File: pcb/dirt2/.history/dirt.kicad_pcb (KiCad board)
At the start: 2 copper layers, 1 part

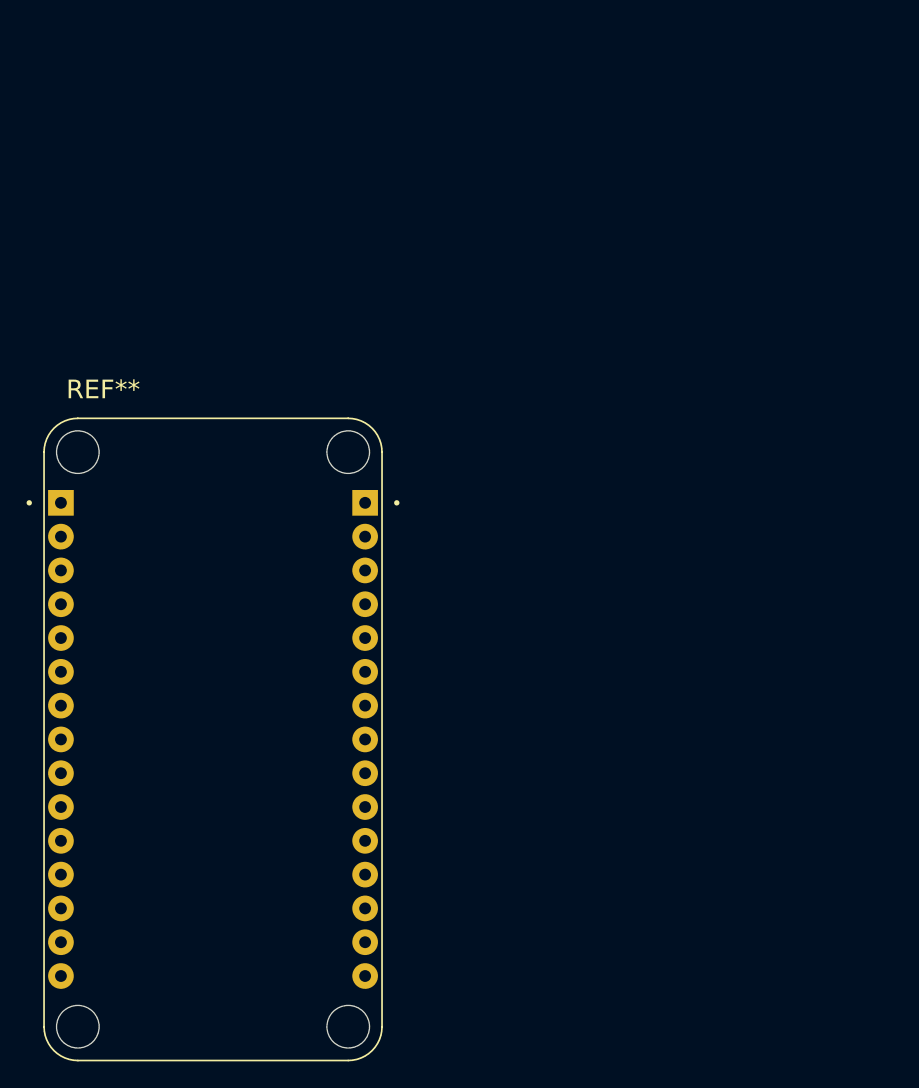
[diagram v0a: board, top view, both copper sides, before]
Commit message: i created some edits and added the zine
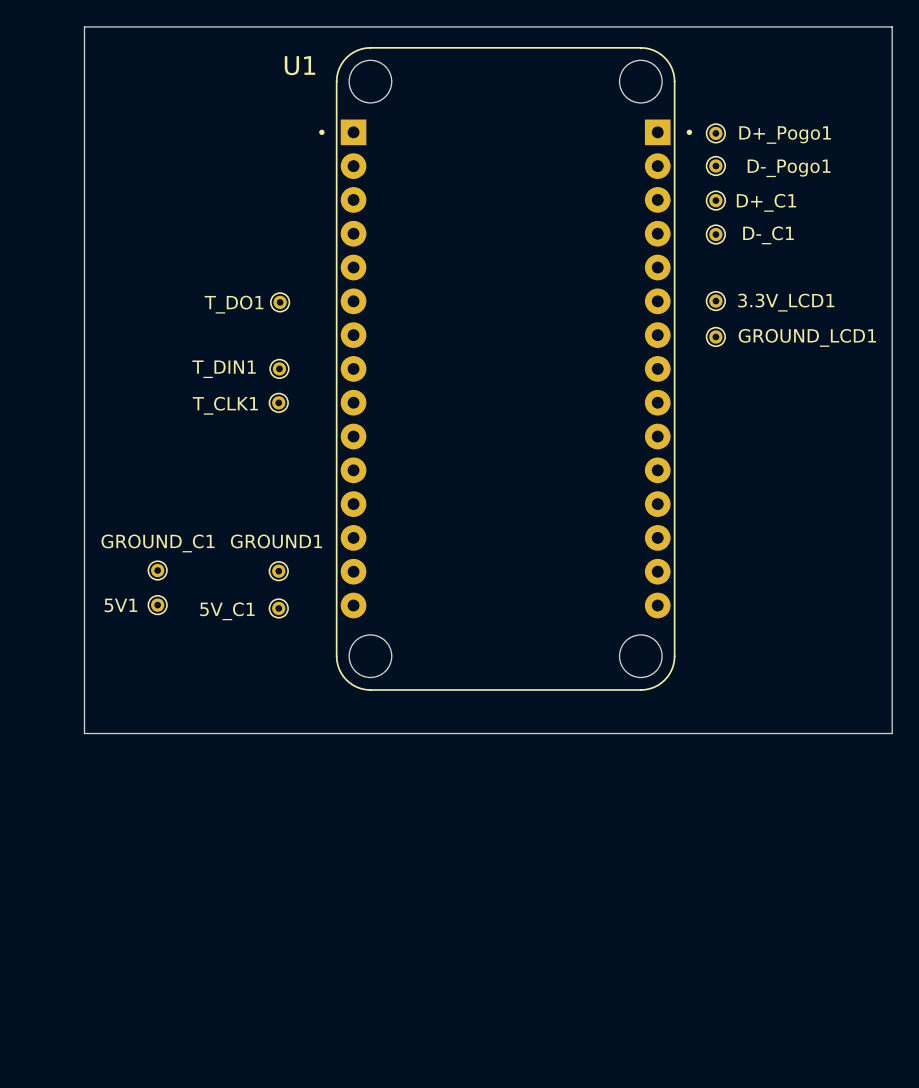
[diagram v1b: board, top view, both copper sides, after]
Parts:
- removed REF**: SEEED_113990105, esp8622footprint:SEEED_113990105
- added 3.3V_LCD1: 3.3V Output to LCD, TestPoint:TestPoint_THTPad_D1.0mm_Drill0.5mm, F.Cu at (174.9, 58.8)
- added 5V1: 5V Output from Pogo, TestPoint:TestPoint_THTPad_D1.0mm_Drill0.5mm, F.Cu at (133.0, 81.6)
- added 5V_C1: 5V Input USB C, TestPoint:TestPoint_THTPad_D1.0mm_Drill0.5mm, F.Cu at (142.1, 81.8)
- added D+_C1: D+ FROM USB C, TestPoint:TestPoint_THTPad_D1.0mm_Drill0.5mm, F.Cu at (174.9, 51.2)
- added D+_Pogo1: D+ FROM Pogo, TestPoint:TestPoint_THTPad_D1.0mm_Drill0.5mm, F.Cu at (174.9, 46.1)
- added D-_C1: D- FROM USB C, TestPoint:TestPoint_THTPad_D1.0mm_Drill0.5mm, F.Cu at (174.9, 53.8)
- added D-_Pogo1: D- FROM Pogo, TestPoint:TestPoint_THTPad_D1.0mm_Drill0.5mm, F.Cu at (174.9, 48.6)
- added GROUND1: GND from Pogo, TestPoint:TestPoint_THTPad_D1.0mm_Drill0.5mm, F.Cu at (142.1, 79.0)
- added GROUND_C1: GND from USB C, TestPoint:TestPoint_THTPad_D1.0mm_Drill0.5mm, F.Cu at (133.0, 79.0)
- added GROUND_LCD1: GND to LCD, TestPoint:TestPoint_THTPad_D1.0mm_Drill0.5mm, F.Cu at (174.9, 61.5)
- added T_CLK1: TestPoint, TestPoint:TestPoint_THTPad_D1.0mm_Drill0.5mm, F.Cu at (142.1, 66.4)
- added T_DIN1: TestPoint, TestPoint:TestPoint_THTPad_D1.0mm_Drill0.5mm, F.Cu at (142.2, 63.9)
- added T_DO1: TestPoint, TestPoint:TestPoint_THTPad_D1.0mm_Drill0.5mm, F.Cu at (142.2, 58.9)
- added U1: ~, esp8622footprint:SEEED_113990105, F.Cu at (159.2, 63.9)
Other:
- board outline added: 60.7 x 53.1 mm
